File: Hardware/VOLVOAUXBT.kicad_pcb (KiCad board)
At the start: 2 copper layers, 100 x 35 mm, 66 parts, among them J1 10118193-0001LF, J10 Conn_01x02_Pin, J11 Conn_01x02_Pin, J12 Conn_01x05_Pin, J13 Conn_01x05_Pin, J14 Conn_01x05_Pin, J15 Conn_01x02_Pin, J16 Conn_01x02_Pin, J17 Conn_01x01_Pin, J18 Conn_01x02_Pin, J19 Conn_01x01_Pin, J2 10118193-0001LF, J3 F52R-1A7H1-11018, J4 Conn_01x18_Pin, J5 Conn_01x18_Pin, J6 F52R-1A7H1-11018, J7 Conn_01x18_Pin, J8 U_FL-R-SMT_10_, J9 Conn_01x02_Pin, U1 SGM2212-3.3, U2 SGM2212-3.3, U3 TJA1027T_20_118, U4 ESP32-MINI-1, U5 TJA1027T_20_118, U6 SN74AHCT157PWR, U7 CP2102N-Axx-xQFN20

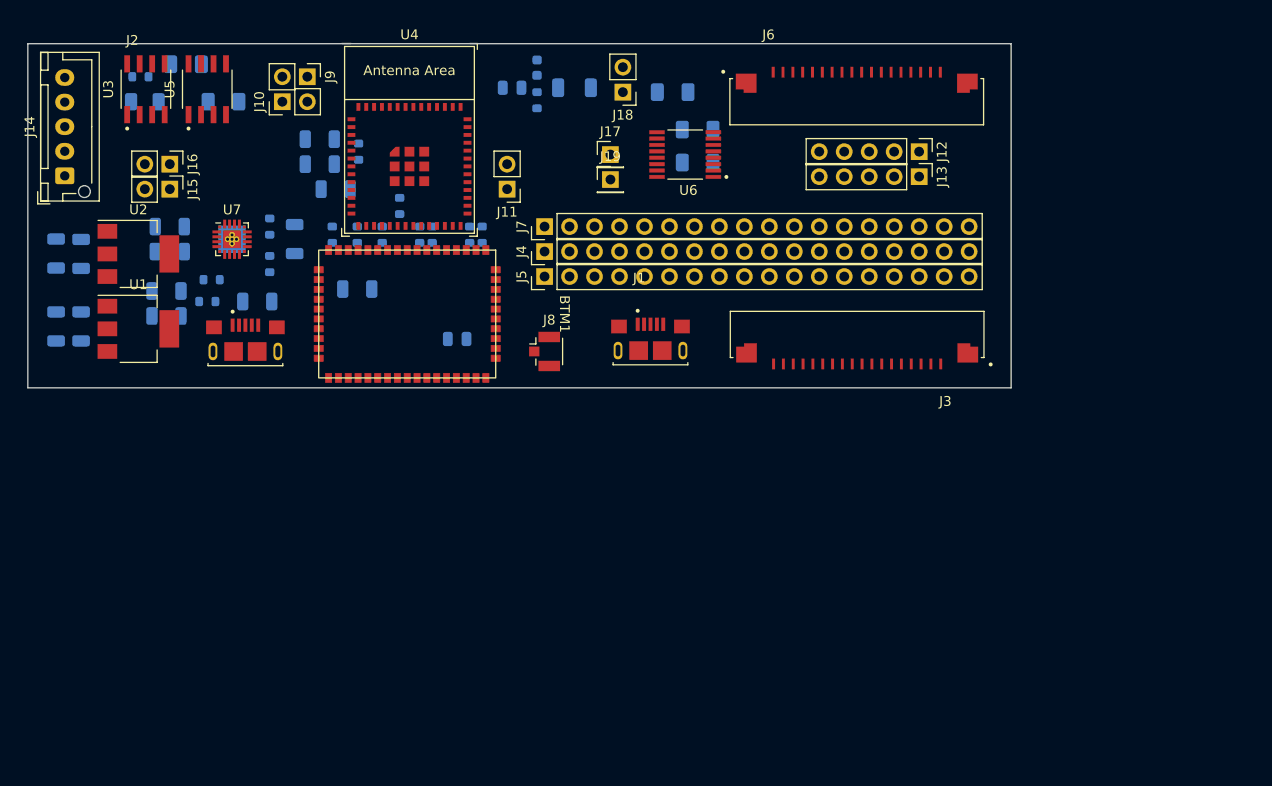
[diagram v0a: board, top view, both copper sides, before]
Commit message: Before swap to wroom
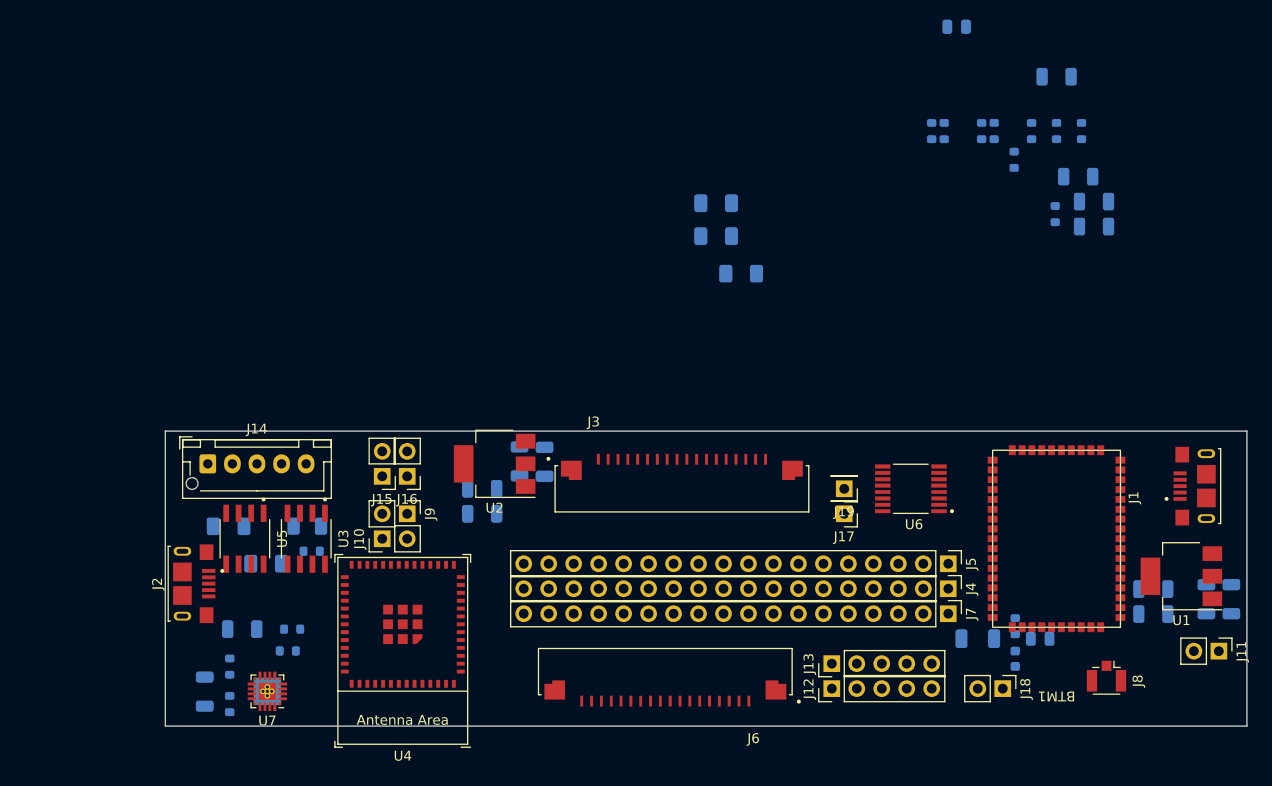
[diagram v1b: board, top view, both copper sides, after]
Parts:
- moved C2 122.7 mm to (161.3, 139.5), turned to -90 degrees
- moved C1 117.8 mm to (158.8, 139.5), turned to -90 degrees
- moved U1 109.0 mm to (156.2, 137.2), turned to 180 degrees
- moved C4 105.6 mm to (153.3, 141.0), turned to 0 degrees
- moved C3 104.1 mm to (153.3, 138.5), turned to 0 degrees
- moved J11 86.3 mm to (160.0, 144.8), turned to -90 degrees
- moved C10 79.2 mm to (147.3, 101.6), turned to 0 degrees
- moved C11 78.8 mm to (147.3, 99.1), turned to 0 degrees
- moved C20 77.6 mm to (141.8, 143.5), turned to 180 degrees
- moved C21 77.3 mm to (139.3, 145.6), turned to -90 degrees
- moved R10 76.9 mm to (146.1, 91.9), turned to -90 degrees
- moved C14 75.5 mm to (145.7, 96.5), turned to 0 degrees
- moved C17 74.3 mm to (143.5, 86.4), turned to 0 degrees
- moved R12 72.3 mm to (139.3, 142.2), turned to -90 degrees
- moved J18 71.9 mm to (138.0, 148.6), turned to -90 degrees
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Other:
- board size 100 x 35 mm -> 110 x 30 mm
